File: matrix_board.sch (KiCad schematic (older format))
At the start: 8 parts, among them J1 MATRIX_CONNECTOR, M1 PWR_LED, M2 LED, U1 ATmega328P-AU

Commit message: commit before milling
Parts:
- C1: footprint kicad_fab:fab-C1206 -> fab:fab-C1206
- JP1: footprint kicad_fab:fab-2X03SMD -> fab:fab-2X03SMD
- M1: footprint kicad_fab:fab-LED1206 -> fab:fab-LCC16
- M2: footprint kicad_fab:fab-LED1206 -> fab:fab-LCC16; symbol kicad_fab:LED -> matrix_board-rescue:LED-kicad_fab
- R1: footprint kicad_fab:fab-R1206 -> fab:fab-R1206
- R2: footprint kicad_fab:fab-R1206 -> fab:fab-R1206; symbol kicad_fab:RES-US1206 -> matrix_board-rescue:RES-US1206-kicad_fab
- U1: footprint Package_QFP:TQFP-32_7x7mm_P0.8mm -> fab:fab-TQFP32-08THIN; symbol MCU_Microchip_ATmega:ATmega328P-AU -> matrix_board-rescue:ATmega328P-AU-MCU_Microchip_ATmega
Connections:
- net labels removed: GND
- no-connect marks 7 -> 8
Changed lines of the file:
@@
 $EndDescr
 $Comp
-L MCU_Microchip_ATmega:ATmega328P-AU U1
+L matrix_board-rescue:ATmega328P-AU-MCU_Microchip_ATmega U1
 U 1 1 5C09DA73
 P 3550 3250
 F 0 "U1" H 3550 1664 50  0000 C CNN
 F 1 "ATmega328P-AU" H 3550 1573 50  0000 C CNN
-F 2 "Package_QFP:TQFP-32_7x7mm_P0.8mm" H 3550 3250 50  0001 C CIN
+F 2 "fab:fab-TQFP32-08THIN" H 3550 3250 50  0001 C CIN
 F 3 "http://ww1.microchip.com/downloads/en/DeviceDoc/ATmega328_P%20AVR%20MCU%20with%20picoPower%20Technology%20Data%20Sheet%2040001984A.pdf" H 3550 3250 50  0001 C CNN
 	1    3550 3250
@@
 F 0 "M1" V 5604 3200 45  0000 C CNN
 F 1 "PWR_LED" V 5520 3200 45  0000 C CNN
-F 2 "kicad_fab:fab-LED1206" H 5430 3300 20  0001 C CNN
+F 2 "fab:fab-LCC16" H 5430 3300 20  0001 C CNN
 F 3 "" H 5400 3150 50  0001 C CNN
 	1    5400 3150
@@
 F 0 "R1" H 5000 3344 45  0000 C CNN
 F 1 "499" H 5000 3260 45  0000 C CNN
-F 2 "kicad_fab:fab-R1206" H 5030 3300 20  0001 C CNN
+F 2 "fab:fab-R1206" H 5030 3300 20  0001 C CNN
 F 3 "" H 5000 3150 50  0001 C CNN
 	1    5000 3150
@@
 F 0 "C1" H 5200 3904 45  0000 C CNN
 F 1 "1uF" H 5200 3820 45  0000 C CNN
-F 2 "kicad_fab:fab-C1206" H 5180 3800 20  0001 C CNN
+F 2 "fab:fab-C1206" H 5180 3800 20  0001 C CNN
 F 3 "" H 5150 3650 50  0001 C CNN
 	1    5150 3650
@@
 LAT
 Text GLabel 5450 2600 2    50   Input ~ 0
-GND
+GROUND
 $Comp
 L matrix_board-rescue:PINHD-2X3-SMD-fab JP1
@@
 F 0 "JP1" H 1800 3354 45  0000 C CNN
 F 1 "ISP" H 1800 3270 45  0000 C CNN
-F 2 "kicad_fab:fab-2X03SMD" H 1780 3150 20  0001 C CNN
+F 2 "fab:fab-2X03SMD" H 1780 3150 20  0001 C CNN
 F 3 "" H 1750 3000 50  0001 C CNN
 	1    1750 3000
@@
 Text GLabel 4150 2350 2    50   Input ~ 0
 MOSI
-Text GLabel 4150 2650 2    50   Input ~ 0
+Text GLabel 4150 2050 2    50   Input ~ 0
 CLK
 Text GLabel 4150 3550 2    50   Input ~ 0
@@
 Text GLabel 4150 3250 2    50   Input ~ 0
 D
-Text GLabel 4150 3750 2    50   Input ~ 0
+Text GLabel 4150 3950 2    50   Input ~ 0
 R1
-Text GLabel 4150 3850 2    50   Input ~ 0
+Text GLabel 4150 4050 2    50   Input ~ 0
 G1
-Text GLabel 4150 3950 2    50   Input ~ 0
+Text GLabel 4150 4150 2    50   Input ~ 0
 B1
-Text GLabel 4150 4050 2    50   Input ~ 0
+Text GLabel 4150 4250 2    50   Input ~ 0
 R2
-Text GLabel 4150 4150 2    50   Input ~ 0
+Text GLabel 4150 4350 2    50   Input ~ 0
 G2
 Text GLabel 4150 4450 2    50   Input ~ 0
 B2
-Text GLabel 4150 4250 2    50   Input ~ 0
+Text GLabel 4150 2250 2    50   Input ~ 0
 LAT
-Text GLabel 4150 4350 2    50   Input ~ 0
+Text GLabel 4150 2150 2    50   Input ~ 0
 OE
 $Comp
-L kicad_fab:RES-US1206 R2
+L matrix_board-rescue:RES-US1206-kicad_fab R2
 U 1 1 5C0D044E
 P 5000 4050
 F 0 "R2" H 5000 4244 45  0000 C CNN
 F 1 "RES-US1206" H 5000 4160 45  0000 C CNN
-F 2 "kicad_fab:fab-R1206" H 5030 4200 20  0001 C CNN
+F 2 "fab:fab-R1206" H 5030 4200 20  0001 C CNN
 F 3 "" H 5000 4050 50  0001 C CNN
 	1    5000 4050
@@
 $EndComp
 $Comp
-L kicad_fab:LED M2
+L matrix_board-rescue:LED-kicad_fab M2
 U 1 1 5C0D0507
 P 5400 4050
 F 0 "M2" V 5604 4100 45  0000 C CNN
 F 1 "LED" V 5520 4100 45  0000 C CNN
-F 2 "kicad_fab:fab-LED1206" H 5430 4200 20  0001 C CNN
+F 2 "fab:fab-LCC16" H 5430 4200 20  0001 C CNN
 F 3 "" H 5400 4050 50  0001 C CNN
 	1    5400 4050
@@
 Text GLabel 5500 4050 2    50   Input ~ 0
 GROUND
-Text GLabel 4150 2250 2    50   Input ~ 0
+Text GLabel 4150 3350 2    50   Input ~ 0
 TEST
-NoConn ~ 4150 2050
-NoConn ~ 4150 2150
-NoConn ~ 4150 3350
 NoConn ~ 4150 3450
 NoConn ~ 2950 2350
 NoConn ~ 2950 2250
 NoConn ~ 2950 2050
+NoConn ~ 4150 2650
+NoConn ~ 4150 2750
+NoConn ~ 4150 3750
+NoConn ~ 4150 3850
 $EndSCHEMATC

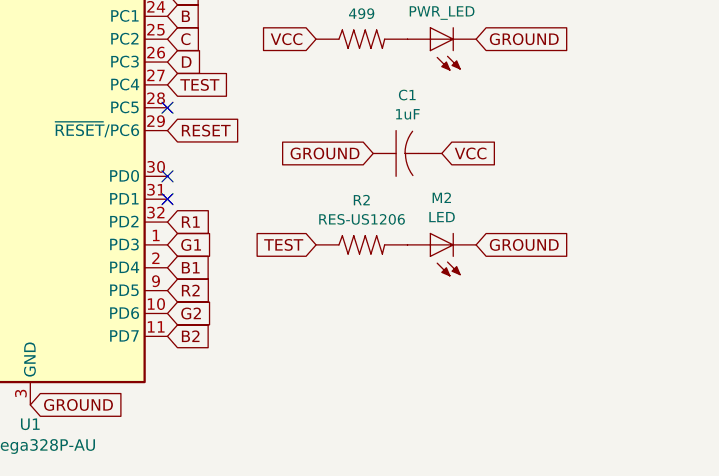
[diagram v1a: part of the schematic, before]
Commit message: added new board design. hope it works
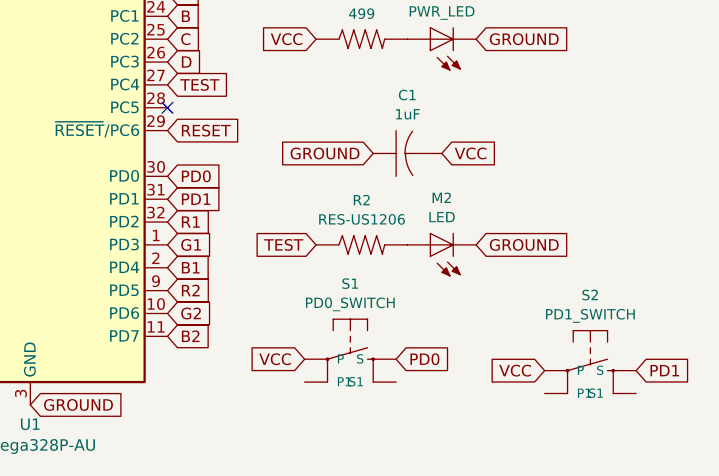
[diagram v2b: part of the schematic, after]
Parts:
- added S1: PD0_SWITCH, fab:fab-6MM_SWITCH, symbol kicad_fab:6MM_SWITCH6MM_SWITCH
- added S2: PD1_SWITCH, fab:fab-6MM_SWITCH, symbol kicad_fab:6MM_SWITCH6MM_SWITCH
- M1, M2: footprint fab:fab-LCC16 -> fab:fab-LED1206
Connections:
- net VCC: now also S1.1 (P), S2.1 (P)
- net PD0: now reaches U1.30 (PD0)
- net PD0: now also S1.3 (S)
- net PD1: now reaches U1.31 (PD1)
- net PD1: now also S2.3 (S)
- no-connect marks 8 -> 6
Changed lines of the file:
@@
 F 0 "M1" V 5604 3200 45  0000 C CNN
 F 1 "PWR_LED" V 5520 3200 45  0000 C CNN
-F 2 "fab:fab-LCC16" H 5430 3300 20  0001 C CNN
+F 2 "fab:fab-LED1206" H 5430 3300 20  0001 C CNN
 F 3 "" H 5400 3150 50  0001 C CNN
 	1    5400 3150
@@
 F 0 "M2" V 5604 4100 45  0000 C CNN
 F 1 "LED" V 5520 4100 45  0000 C CNN
-F 2 "fab:fab-LCC16" H 5430 4200 20  0001 C CNN
+F 2 "fab:fab-LED1206" H 5430 4200 20  0001 C CNN
 F 3 "" H 5400 4050 50  0001 C CNN
 	1    5400 4050
@@
 NoConn ~ 4150 2650
 NoConn ~ 4150 2750
-NoConn ~ 4150 3750
-NoConn ~ 4150 3850
+Text GLabel 4150 3750 2    50   Input ~ 0
+PD0
+Text GLabel 4150 3850 2    50   Input ~ 0
+PD1
+$Comp
+L kicad_fab:6MM_SWITCH6MM_SWITCH S1
+U 1 1 5C15CBC9
+P 4950 4550
+F 0 "S1" V 4621 4550 45  0000 C CNN
+F 1 "PD0_SWITCH" V 4705 4550 45  0000 C CNN
+F 2 "fab:fab-6MM_SWITCH" H 4980 4700 20  0001 C CNN
+F 3 "" H 4950 4550 50  0001 C CNN
+	1    4950 4550
+	0    1    1    0
+$EndComp
+$Comp
+L kicad_fab:6MM_SWITCH6MM_SWITCH S2
+U 1 1 5C15CC59
+P 6000 4600
+F 0 "S2" V 5671 4600 45  0000 C CNN
+F 1 "PD1_SWITCH" V 5755 4600 45  0000 C CNN
+F 2 "fab:fab-6MM_SWITCH" H 6030 4750 20  0001 C CNN
+F 3 "" H 6000 4600 50  0001 C CNN
+	1    6000 4600
+	0    1    1    0
+$EndComp
+Text GLabel 5150 4550 2    50   Input ~ 0
+PD0
+Text GLabel 6200 4600 2    50   Input ~ 0
+PD1
+Text GLabel 4750 4550 0    50   Input ~ 0
+VCC
+Text GLabel 5800 4600 0    50   Input ~ 0
+VCC
 $EndSCHEMATC

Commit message: remade board to be bigger
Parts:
- added M3: PINHD-2X2-SMD, fab:fab-2X02SMD, symbol fab:PINHD-2X2-SMD
- S1, S2: symbol kicad_fab:6MM_SWITCH6MM_SWITCH -> matrix_board-rescue:6MM_SWITCH6MM_SWITCH-kicad_fab
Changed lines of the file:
@@
 PD1
 $Comp
-L kicad_fab:6MM_SWITCH6MM_SWITCH S1
+L matrix_board-rescue:6MM_SWITCH6MM_SWITCH-kicad_fab S1
 U 1 1 5C15CBC9
 P 4950 4550
@@
 $EndComp
 $Comp
-L kicad_fab:6MM_SWITCH6MM_SWITCH S2
+L matrix_board-rescue:6MM_SWITCH6MM_SWITCH-kicad_fab S2
 U 1 1 5C15CC59
 P 6000 4600
@@
 Text GLabel 5800 4600 0    50   Input ~ 0
 VCC
+$Comp
+L fab:PINHD-2X2-SMD M3
+U 1 1 5C1691BE
+P 5000 5250
+F 0 "M3" H 4950 5604 45  0000 C CNN
+F 1 "PINHD-2X2-SMD" H 4950 5520 45  0000 C CNN
+F 2 "fab:fab-2X02SMD" H 5030 5400 20  0001 C CNN
+F 3 "" H 5000 5250 50  0001 C CNN
+	1    5000 5250
+	1    0    0    -1
+$EndComp
+Text GLabel 4800 5150 0    50   Input ~ 0
+VCC
+Text GLabel 5100 5150 2    50   Input ~ 0
+GROUND
+Text GLabel 4800 5250 0    50   Input ~ 0
+VCC
+Text GLabel 5100 5250 2    50   Input ~ 0
+GROUND
 $EndSCHEMATC

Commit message: updated board with more components so it'll work
added pull up resistor on reset and clock on xtal, also moved capacitor closer to chip
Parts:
- added M4: RESONATOR, fab:fab-EFOBM, symbol fab:RESONATOR
- added R3: 10k, fab:fab-R1206, symbol fab:RES-US1206
- J1: footprint Connector_PinHeader_2.00mm:PinHeader_2x08_P2.00mm_Vertical_SMD -> fab:fab-2X08SMD
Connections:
- net labels added: XTAL1, XTAL2
- no-connect marks 6 -> 4
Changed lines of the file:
@@
 $EndDescr
-$Comp
-L matrix_board-rescue:ATmega328P-AU-MCU_Microchip_ATmega U1
-U 1 1 5C09DA73
-P 3550 3250
-F 0 "U1" H 3550 1664 50  0000 C CNN
-F 1 "ATmega328P-AU" H 3550 1573 50  0000 C CNN
-F 2 "fab:fab-TQFP32-08THIN" H 3550 3250 50  0001 C CIN
-F 3 "http://ww1.microchip.com/downloads/en/DeviceDoc/ATmega328_P%20AVR%20MCU%20with%20picoPower%20Technology%20Data%20Sheet%2040001984A.pdf" H 3550 3250 50  0001 C CNN
-	1    3550 3250
-	1    0    0    -1
-$EndComp
 $Comp
 L matrix_board-rescue:LED-fab M1
@@
 F 0 "J1" H 5200 2717 50  0000 C CNN
 F 1 "MATRIX_CONNECTOR" H 5200 2626 50  0000 C CNN
-F 2 "Connector_PinHeader_2.00mm:PinHeader_2x08_P2.00mm_Vertical_SMD" H 5150 2200 50  0001 C CNN
+F 2 "fab:fab-2X08SMD" H 5150 2200 50  0001 C CNN
 F 3 "~" H 5150 2200 50  0001 C CNN
 	1    5150 2200
@@
 NoConn ~ 2950 2250
 NoConn ~ 2950 2050
-NoConn ~ 4150 2650
-NoConn ~ 4150 2750
 Text GLabel 4150 3750 2    50   Input ~ 0
 PD0
@@
 Text GLabel 5100 5250 2    50   Input ~ 0
 GROUND
+$Comp
+L fab:RES-US1206 R3
+U 1 1 5C16F8E5
+P 6200 3650
+F 0 "R3" H 6200 3844 45  0000 C CNN
+F 1 "10k" H 6200 3760 45  0000 C CNN
+F 2 "fab:fab-R1206" H 6230 3800 20  0001 C CNN
+F 3 "" H 6200 3650 50  0001 C CNN
+	1    6200 3650
+	1    0    0    -1
+$EndComp
+Text GLabel 6000 3650 0    50   Input ~ 0
+VCC
+Text GLabel 6400 3650 2    50   Input ~ 0
+RESET
+$Comp
+L matrix_board-rescue:ATmega328P-AU-MCU_Microchip_ATmega U1
+U 1 1 5C09DA73
+P 3550 3250
+F 0 "U1" H 3550 1664 50  0000 C CNN
+F 1 "ATmega328P-AU" H 3550 1573 50  0000 C CNN
+F 2 "fab:fab-TQFP32-08THIN" H 3550 3250 50  0001 C CIN
+F 3 "http://ww1.microchip.com/downloads/en/DeviceDoc/ATmega328_P%20AVR%20MCU%20with%20picoPower%20Technology%20Data%20Sheet%2040001984A.pdf" H 3550 3250 50  0001 C CNN
+	1    3550 3250
+	1    0    0    -1
+$EndComp
+Text GLabel 4150 2650 2    50   Input ~ 0
+XTAL1
+Text GLabel 4150 2750 2    50   Input ~ 0
+XTAL2
+$Comp
+L fab:RESONATOR M4
+U 1 1 5C17B852
+P 6700 2350
+F 0 "M4" H 6700 2604 45  0000 C CNN
+F 1 "RESONATOR" H 6700 2520 45  0000 C CNN
+F 2 "fab:fab-EFOBM" H 6730 2500 20  0001 C CNN
+F 3 "" H 6700 2350 50  0001 C CNN
+	1    6700 2350
+	1    0    0    -1
+$EndComp
+Text GLabel 6400 2350 0    50   Input ~ 0
+XTAL1
+Text GLabel 7000 2350 2    50   Input ~ 0
+XTAL2
+Text GLabel 6700 2650 3    50   Input ~ 0
+GROUND
 $EndSCHEMATC
